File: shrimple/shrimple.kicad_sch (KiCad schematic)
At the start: 108 parts, among them U3 Sparkfun_Pro_Micro

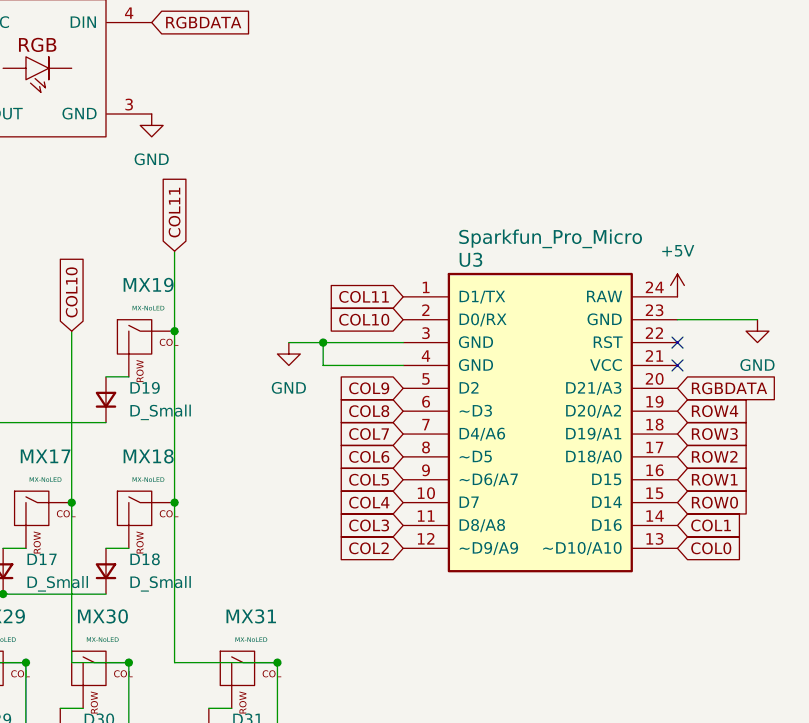
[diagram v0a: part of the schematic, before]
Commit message: added LED, routing attempt the first
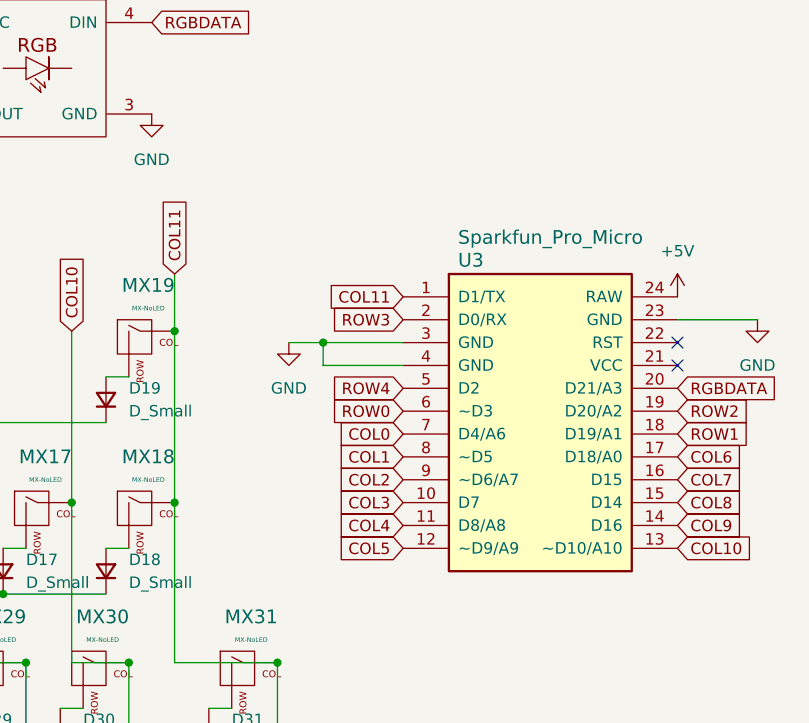
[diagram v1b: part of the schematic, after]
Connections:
- net COL0: now also U3.7 (D4/A6); no longer U3.13 (~D10/A10)
- net COL1: now also U3.8 (~D5); no longer U3.14 (D16)
- net COL10: now also U3.13 (~D10/A10); no longer U3.2 (D0/RX)
- net COL2: now also U3.9 (~D6/A7); no longer U3.12 (~D9/A9)
- net COL3: now also U3.10 (D7); no longer U3.11 (D8/A8)
- net COL4: now also U3.11 (D8/A8); no longer U3.10 (D7)
- net COL5: now also U3.12 (~D9/A9); no longer U3.9 (~D6/A7)
- net COL6: now also U3.17 (D18/A0); no longer U3.8 (~D5)
- net COL7: now also U3.16 (D15); no longer U3.7 (D4/A6)
- net COL8: now also U3.15 (D14); no longer U3.6 (~D3)
- net COL9: now also U3.14 (D16); no longer U3.5 (D2)
- net ROW0: now also U3.6 (~D3); no longer U3.15 (D14)
- net ROW1: now also U3.18 (D19/A1); no longer U3.16 (D15)
- net ROW2: now also U3.19 (D20/A2); no longer U3.17 (D18/A0)
- net ROW3: now also U3.2 (D0/RX); no longer U3.18 (D19/A1)
- net ROW4: now also U3.5 (D2); no longer U3.19 (D20/A2)
